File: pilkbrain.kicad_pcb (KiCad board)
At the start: 4 copper layers, 22 x 33 mm, 106 parts, among them CN1 SM02B-SRSS-TB (LF)(SN), SW1 TS24CA, SW3 TS24CA, U1 TYPE-C 16P LTH8.8, U11 TF-123-ARP9H17, U12 SM03B-SRSS-TB(LF)(SN)(P), U13 ESP32-S3, U2 XL-1005UWC_C20613596, U3 SSP7615-33DFR, U4 BQ24073RGT, U5 XL-1005UWC_C20613596, U6 XL-1005UWC_C20613596, U7 AP2552FDC-7, U8 MAX98357AEWL+T, U9 SSP7615-33DFR, Y1 XO-40M, Y2 XO-32K

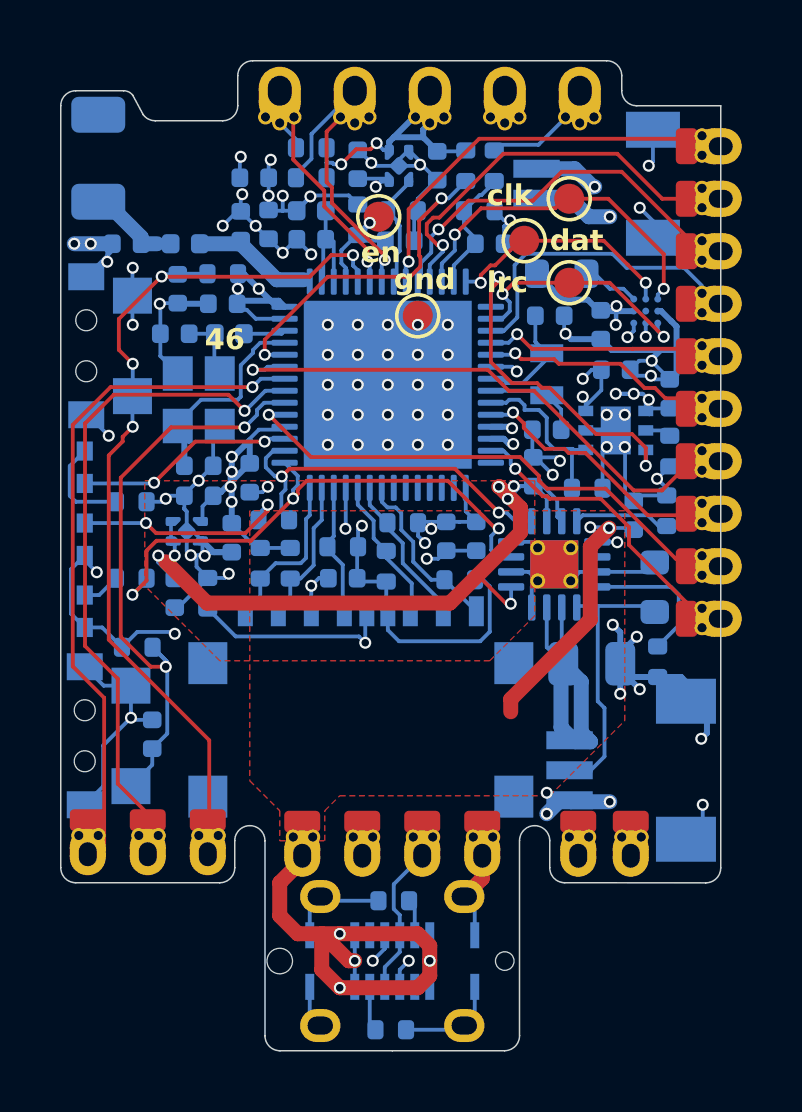
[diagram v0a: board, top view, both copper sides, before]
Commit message: another element swappage
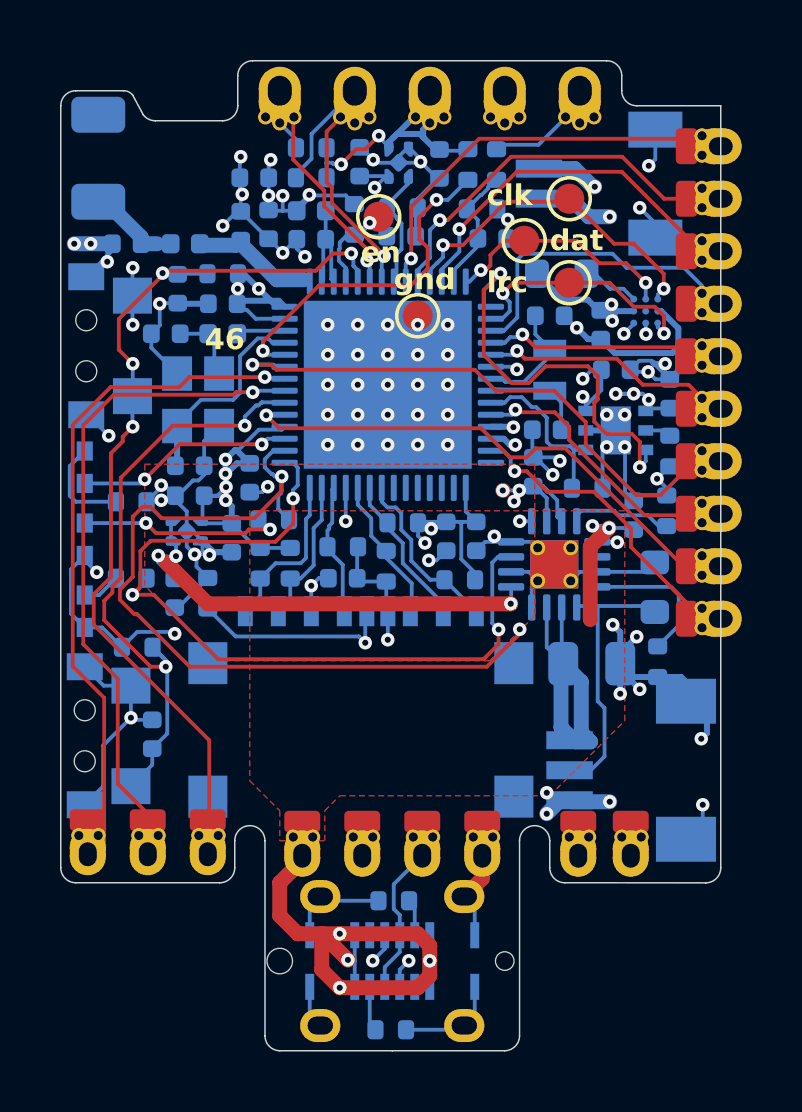
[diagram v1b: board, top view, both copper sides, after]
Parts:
- moved C3 0.30 mm to (101.5, 53.0)
- moved C7 0.30 mm to (100.7, 47.6)
- moved C8 0.30 mm to (101.5, 52.0)
- moved L3 0.22 mm to (102.6, 47.6)
- moved C17 0.20 mm to (111.6, 44.4)
- moved Y2 0.18 mm to (113.5, 48.8)
- moved C21 0.16 mm to (108.5, 44.4)
- moved R5 0.11 mm to (111.2, 43.4)
- moved R7 0.11 mm to (107.0, 43.8)
- moved C14 0.11 mm to (107.2, 41.9)
- moved U3 0.10 mm to (108.5, 41.9)
- moved R18 0.10 mm to (108.6, 43.4)
- moved C15 0.10 mm to (109.8, 41.9)
- moved R3 0.09 mm to (111.7, 42.0)
- moved R27 0.08 mm to (110.8, 42.0)
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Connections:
- U13 pad 10: /EXTIO_8 -> /EXTIO_9
- U13 pad 11: /EXTIO_9 -> /I2S_CLK
- U13 pad 12: /I2S_CLK -> /EXTIO_8
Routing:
- net /BQ_CHG: track 25.8 -> 41.2 mm, vias 2 -> 3
- net /WS2812_VDD: track 22.2 -> 31.6 mm
- net GND: track 106.7 -> 100.0 mm, vias 71 -> 70
- net +3.3V: track 64.9 -> 58.4 mm
- net +4V: track 42.7 -> 36.3 mm
- net VBUS: track 30.1 -> 25.8 mm
- net /BQ_PGOOD: track 31.0 -> 34.7 mm
- net /PERIPH_FAULT: track 11.5 -> 13.7 mm
- net /EXTIO_9: track 14.7 -> 13.5 mm
- net Net-(U13-XTAL_N): track 7.25 -> 6.25 mm
- net /EXTIO_8: track 12.4 -> 11.6 mm
- net /3V3_MEAS: track 11.0 -> 11.6 mm
- net /BUT2: track 20.0 -> 20.5 mm
